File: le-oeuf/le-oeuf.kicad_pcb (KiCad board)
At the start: 2 copper layers, 215.1 x 81.2 mm, 80 parts, among them J1 S2B-PH-K-S, SW1 PG1425, SW10 PG1425, SW11 PG1425, SW12 PG1425, SW13 PG1425, SW14 PG1425, SW15 PG1425, SW16 PG1425, SW17 PG1425, SW18 PG1425, SW19 PG1425, SW2 PG1425, SW20 PG1425, SW21 PG1425, SW22 PG1425, SW23 PG1425, SW24 PG1425, SW25 PG1425, SW26 PG1425, SW27 PG1425, SW28 PG1425, SW29 PG1425, SW3 PG1425, SW30 PG1425, SW31 PG1425, SW32 PG1425, SW33 PG1425, SW34 PG1425, SW35 PG1425, SW36 PG1425, SW37 PCM12SMTR, SW4 PG1425, SW5 PG1425, SW6 PG1425, SW7 PG1425, SW8 PG1425, SW9 PG1425, U1 Seeeduino Xiao nRF52840, U2 74HC595D,118

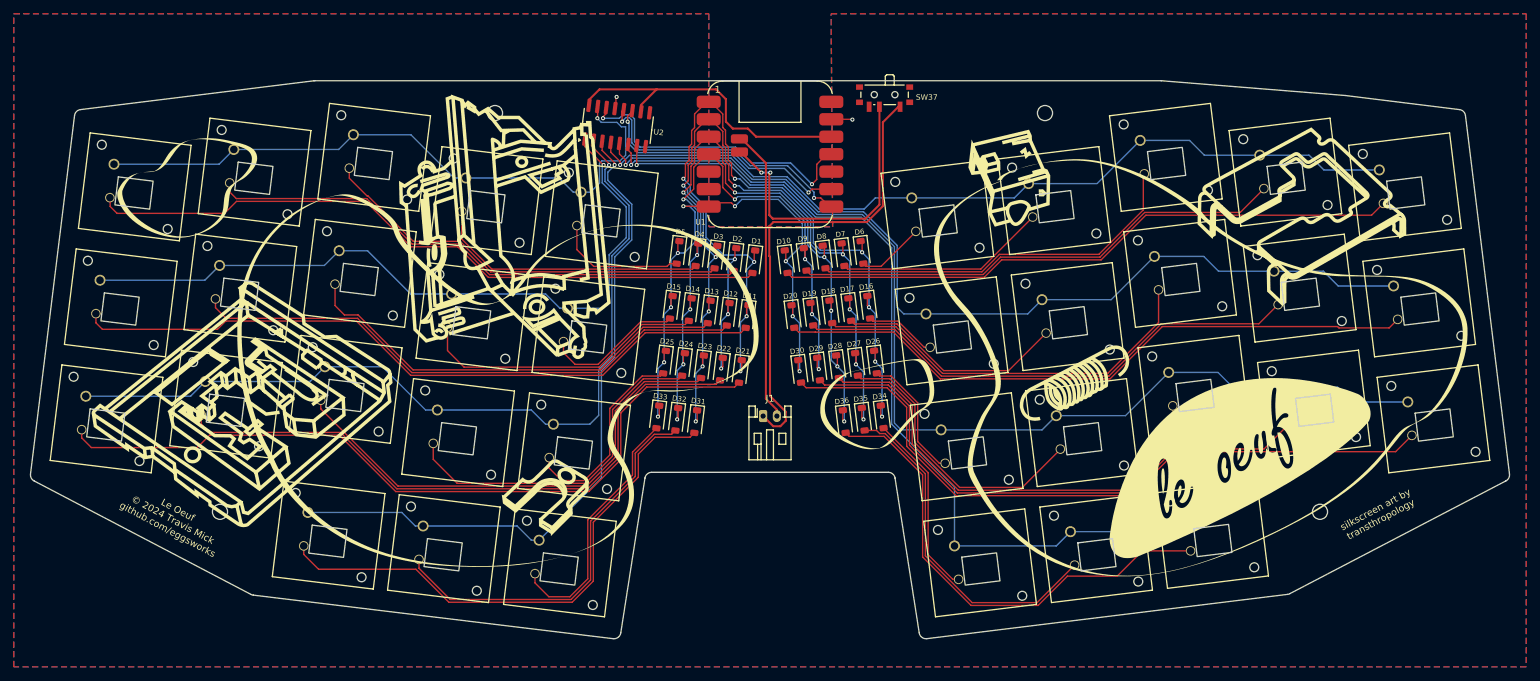
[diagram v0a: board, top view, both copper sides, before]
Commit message: do not push this commit
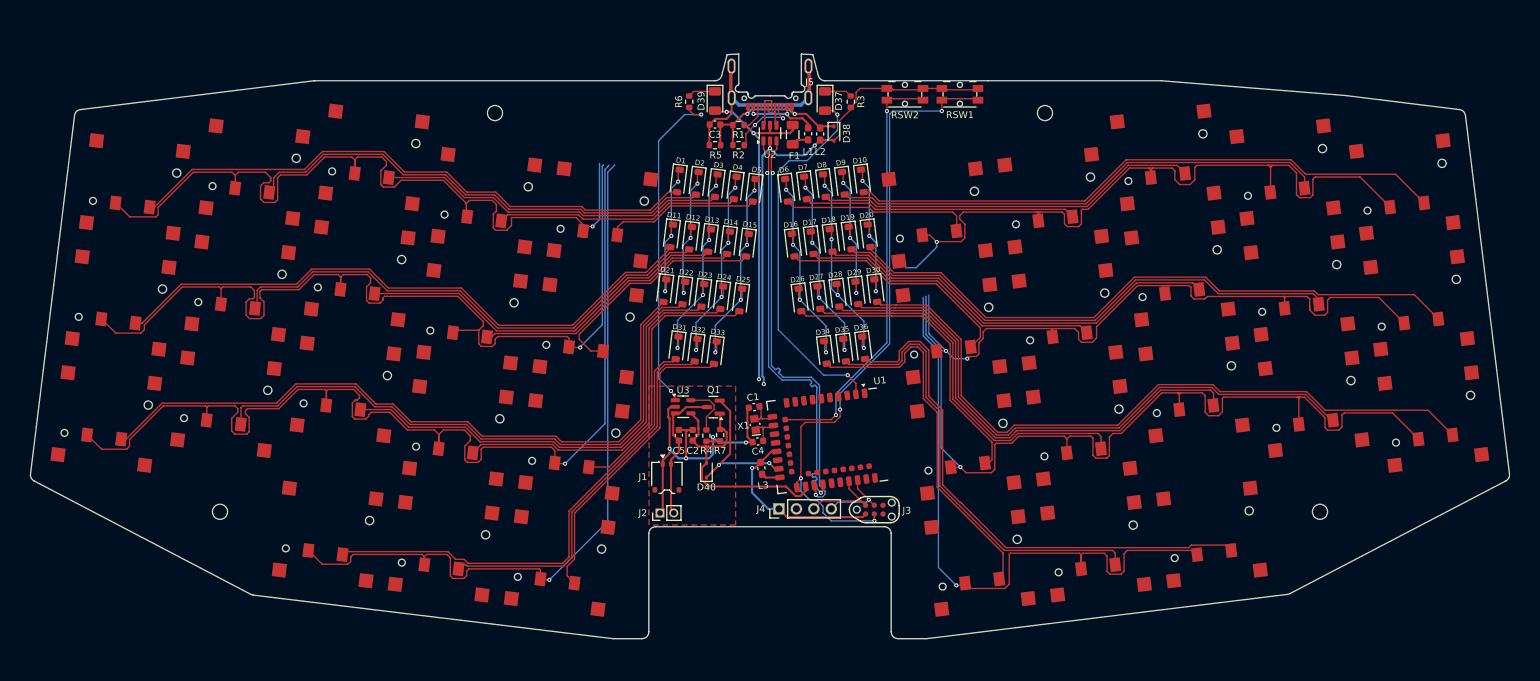
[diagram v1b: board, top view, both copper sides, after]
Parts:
- removed the SW34 at (169.5, 114.4)
- removed SW37: PCM12SMTR, Button_Switch_SMD:SW_SPDT_PCM12
- added C1: 12pF, Capacitor_SMD:C_0603_1608Metric, F.Cu at (136.6, 91.8)
- added C2: 4.7uF, Capacitor_SMD:C_0603_1608Metric, F.Cu at (127.7, 95.9)
- added C3: 100nF, Capacitor_SMD:C_0603_1608Metric, F.Cu at (130.9, 50.7)
- added C4: 12pF, Capacitor_SMD:C_0603_1608Metric, F.Cu at (137.1, 96.8)
- added C5: 4.7uF, Capacitor_SMD:C_0603_1608Metric, F.Cu at (125.7, 95.9)
- added D37: BLUE, LED_SMD:LED_1206_3216Metric, F.Cu at (146.9, 47.3)
- added D38: BSD3C051V, Diode_SMD:D_SOD-323, F.Cu at (148.2, 52.0)
- added D39: RED, LED_SMD:LED_1206_3216Metric, F.Cu at (130.9, 47.3)
- added D40: 1N5819, Diode_SMD:D_SOD-323, F.Cu at (129.7, 101.0)
- added F1: 500mA, Fuse:Fuse_1206_3216Metric, F.Cu at (142.2, 52.2)
- added J2: Battery, Connector_PinHeader_2.00mm:PinHeader_1x02_P2.00mm_Vertical, F.Cu at (122.9, 107.2)
- added J3: TC2030_SWD, PCM_marbastlib-various:CON_TC2030_outlined, F.Cu at (154.1, 106.7)
- added J4: SWD, Connector_PinHeader_2.54mm:PinHeader_1x04_P2.54mm_Vertical, F.Cu at (140.2, 106.6)
- added J5: USB-C Conn, PCM_marbastlib-various:USB_C_Receptacle_HRO_TYPE-C-31-M-14, F.Cu at (138.9, 46.9)
- added L1: HPZ1608U121, Inductor_SMD:L_0603_1608Metric_Pad1.05x0.95mm_HandSolder, F.Cu at (144.5, 52.0)
- added L2: HPZ1608U121, Inductor_SMD:L_0603_1608Metric_Pad1.05x0.95mm_HandSolder, F.Cu at (146.2, 52.1)
- added L3: 10uH, Inductor_SMD:L_0603_1608Metric_Pad1.05x0.95mm_HandSolder, F.Cu at (137.7, 100.7)
- added Q1: AO3407, Package_TO_SOT_SMD:SOT-23, F.Cu at (130.7, 91.8)
- added R1: 5.1K, Resistor_SMD:R_0603_1608Metric, F.Cu at (134.3, 50.8)
- added R2: 5.1K, Resistor_SMD:R_0603_1608Metric, F.Cu at (134.3, 53.7)
- added R3: 1K, Resistor_SMD:R_0603_1608Metric, F.Cu at (150.7, 47.4)
- added R4: 10K, Resistor_SMD:R_0603_1608Metric, F.Cu at (129.7, 95.9)
- added R5: 1M, Resistor_SMD:R_0603_1608Metric, F.Cu at (130.9, 53.7)
- added R6: 1K, Resistor_SMD:R_0603_1608Metric, F.Cu at (127.2, 47.4)
- added R7: 100K, Resistor_SMD:R_0603_1608Metric, F.Cu at (131.7, 95.9)
- added RSW1: SW_PUSH, Button_Switch_SMD:Panasonic_EVQPUL_EVQPUC, F.Cu at (166.5, 46.3)
- added RSW2: SW_PUSH, Button_Switch_SMD:Panasonic_EVQPUL_EVQPUC, F.Cu at (158.5, 46.3)
- added SW36: PG1425, le-oeuf:CPG1316S01D02_mikeholscher, F.Cu at (203.2, 110.3)
- added U3: TP4054, Package_TO_SOT_SMD:SOT-23-5, F.Cu at (126.3, 91.7)
- added X1: 32.768kHz, Crystal:Crystal_SMD_MicroCrystal_CM9V-T1A-2Pin_1.6x1.0mm_HandSoldering, F.Cu at (136.7, 94.3)
- J1: value S2B-PH-K-S -> Battery JST; footprint Connector_JST:JST_PH_S2B-PH-K_1x02_P2.00mm_Horizontal -> Connector_JST:JST_ACH_BM02B-ACHSS-GAN-ETF_1x02-1MP_P1.20mm_Vertical
- SW1, SW10, SW11, SW12, SW13, SW14, SW15, SW16, SW17, SW18, SW19, SW2, SW20, SW21, SW22, SW23, SW24, SW25, SW26, SW27, SW28, SW29, SW3, SW30, SW31, SW32, SW33, SW4, SW5, SW6, SW7, SW8, SW9: footprint le-oeuf:Kailh-PG1425-X-Switch -> le-oeuf:CPG1316S01D02_mikeholscher
- SW34: renamed from SW35; footprint le-oeuf:Kailh-PG1425-X-Switch -> le-oeuf:CPG1316S01D02_mikeholscher
- SW35: renamed from SW36; footprint le-oeuf:Kailh-PG1425-X-Switch -> le-oeuf:CPG1316S01D02_mikeholscher
- U1: value Seeeduino Xiao nRF52840 -> E73-2G4M08S1C-52840; footprint le-oeuf:Xiao_nRF52840_AC_Reflow -> PCM_marbastlib-various:nRF52840_E73-2G4M08S1C
- U2: value 74HC595D,118 -> USBLC6-2SC6; footprint Package_SO:SOIC-16_3.9x9.9mm_P1.27mm -> Package_TO_SOT_SMD:TSOT-23-6
- moved U1 42.6 mm to (148.4, 96.6), turned to -83 degrees
- moved U2 22.2 mm to (138.9, 51.9), turned to 90 degrees
- moved SW34 17.0 mm to (169.4, 114.5)
- moved SW35 17.0 mm to (186.3, 112.4)
- moved J1 16.6 mm to (123.9, 101.9)
- moved D33 12.5 mm to (131.0, 83.9)
- moved D34 12.5 mm to (147.0, 83.8)
- moved D12 10.4 mm to (127.4, 67.2)
- moved D29 10.4 mm to (151.5, 75.2)
- moved D10 10.4 mm to (152.3, 58.9)
- moved D2 10.4 mm to (128.3, 59.2)
- moved D5 10.4 mm to (136.6, 60.3)
- moved D6 10.4 mm to (141.3, 60.2)
- moved D8 10.4 mm to (146.8, 59.6)
- moved D1 10.4 mm to (125.6, 58.9)
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- renumbered D5 to D1, D6 to D10, D15 to D11, D14 to D12, D12 to D14, D11 to D15, D20 to D16, D19 to D17, D17 to D19, D4 to D2, D16 to D20, D25 to D21, D24 to D22, D22 to D24, D21 to D25, D30 to D26, D29 to D27, D27 to D29, D26 to D30, D32 to D31, D31 to D32, D36 to D35, D35 to D36, D2 to D4, D1 to D5, D10 to D6, D9 to D7, D7 to D9
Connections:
- D1 pad 2: Net-(D5-A) -> Net-(D1-A)
- D10 pad 2: Net-(D6-A) -> Net-(D10-A)
- D11 pad 2: Net-(D15-A) -> Net-(D11-A)
- D12 pad 2: Net-(D14-A) -> Net-(D12-A)
- D14 pad 2: Net-(D12-A) -> Net-(D14-A)
- D15 pad 2: Net-(D11-A) -> Net-(D15-A)
- D16 pad 2: Net-(D20-A) -> Net-(D16-A)
- D17 pad 2: Net-(D19-A) -> Net-(D17-A)
- D19 pad 2: Net-(D17-A) -> Net-(D19-A)
- D2 pad 2: Net-(D4-A) -> Net-(D2-A)
- D20 pad 2: Net-(D16-A) -> Net-(D20-A)
- D21 pad 2: Net-(D25-A) -> Net-(D21-A)
- D22 pad 2: Net-(D24-A) -> Net-(D22-A)
- D24 pad 2: Net-(D22-A) -> Net-(D24-A)
- D25 pad 2: Net-(D21-A) -> Net-(D25-A)
- D26 pad 2: Net-(D30-A) -> Net-(D26-A)
- D27 pad 2: Net-(D29-A) -> Net-(D27-A)
- D29 pad 2: Net-(D27-A) -> Net-(D29-A)
- D30 pad 2: Net-(D26-A) -> Net-(D30-A)
- D31 pad 1: C4 -> C3
- D31 pad 2: Net-(D32-A) -> Net-(D31-A)
- D32 pad 1: C3 -> C2
- D32 pad 2: Net-(D31-A) -> Net-(D32-A)
- D33 pad 1: C5 -> C1
- D34 pad 1: C1 -> C5
- D35 pad 1: C3 -> C4
- D36 pad 1: C2 -> C3
- D36 pad 2: Net-(D35-A) (its old number) -> Net-(D36-A)
- D4 pad 2: Net-(D2-A) -> Net-(D4-A)
- D5 pad 2: Net-(D1-A) -> Net-(D5-A)
- D6 pad 2: Net-(D10-A) -> Net-(D6-A)
- D7 pad 2: Net-(D9-A) -> Net-(D7-A)
- D9 pad 2: Net-(D7-A) -> Net-(D9-A)
- J1 pad 1: Net-(J1-Pin_1) -> GND
- J1 pad 2: Net-(J1-Pin_2) -> VBAT
- SW34 pad 2: Net-(D35-A) (its old number) -> Net-(D34-A)
- U1 pad 1: C1 -> unconnected-(U1-P1.11-Pad1)
- U1 pad 10: VCC -> unconnected-(U1-P0.30/AIN6-Pad10)
- U1 pad 11: MOSI -> XL1
- U1 pad 12: unconnected-(U1-P1.14-Pad12) -> SOFT_OFF
- U1 pad 13: SCK -> XL2
- U1 pad 14: CS -> unconnected-(U1-P0.06-Pad14)
- U1 pad 15: Net-(J1-Pin_2) -> unconnected-(U1-P0.05/AIN3-Pad15)
- U1 pad 16: Net-(SW37-B) -> unconnected-(U1-P0.08-Pad16)
- U1 pad 2: C2 -> BLUE_LED
- U1 pad 3: C3 -> unconnected-(U1-P0.03/AIN1-Pad3)
- U1 pad 4: C4 -> unconnected-(U1-P0.28/AIN4-Pad4)
- U1 pad 5: unconnected-(U1-P0.04-Pad5) -> GND
- U1 pad 7: C5 -> unconnected-(U1-P0.02/AIN0-Pad7)
- U1 pad 9: GND -> unconnected-(U1-P0.31/AIN7-Pad9)
- U2 pad 1: R2 -> DATA+
- U2 pad 2: R3 -> GND
- U2 pad 3: R4 -> DATA-
- U2 pad 4: R5 -> USBN
- U2 pad 5: R6 -> VBUS
- U2 pad 6: R7 -> USBP
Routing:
- net GND: track 4.88 -> 120.8 mm, vias 2 -> 7
- net RESET: track 0.00 -> 93.1 mm, vias 0 -> 4
- net VBUS: track 0.00 -> 89.6 mm, vias 0 -> 3
- net Net-(D36-A): track 0.00 -> 78.8 mm
- net C1: track 123.0 -> 54.7 mm, vias 9 -> 7
- net Net-(J1-Pin_1): track 66.9 -> 0.00 mm
- net SOFT_OFF: track 0.00 -> 61.9 mm, vias 0 -> 2
- net DATA-: track 0.00 -> 61.3 mm, vias 0 -> 2
- net DATA+: track 0.00 -> 61.2 mm, vias 0 -> 2
- net C2: track 113.3 -> 53.3 mm, vias 9 -> 7
- net BLUE_LED: track 0.00 -> 54.6 mm, vias 0 -> 2
- net Net-(D35-A) (its old number): track 50.2 -> 0.00 mm
- net C3: track 113.7 -> 63.6 mm, vias 10 -> 8
- net Net-(U3-STAT): track 0.00 -> 48.9 mm, vias 0 -> 2
- net VCC: track 45.6 -> 0.00 mm
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- removed copper zone on B.Cu, net GND
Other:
- board size 215.1 x 81.2 mm -> 215.1 x 85 mm
- board text added: "Le Oeuf v2 © 2024 Travis Mick github.com/eggsworks"
- board text removed: "Le Oeuf © 2024 Travis Mick github.com/eggsworks"
- board text removed: "silkscreen art by transthropology"
